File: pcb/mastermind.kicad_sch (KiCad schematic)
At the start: 14 parts, among them J1 Battery connector, SW1 SW_Push, SW2 SW_Push, SW3 SW_Push, SW4 SW_Push, SW5 SW_Push, SW6 SW_Push, SW7 SW_RST, U1 SuperMini nRF52840

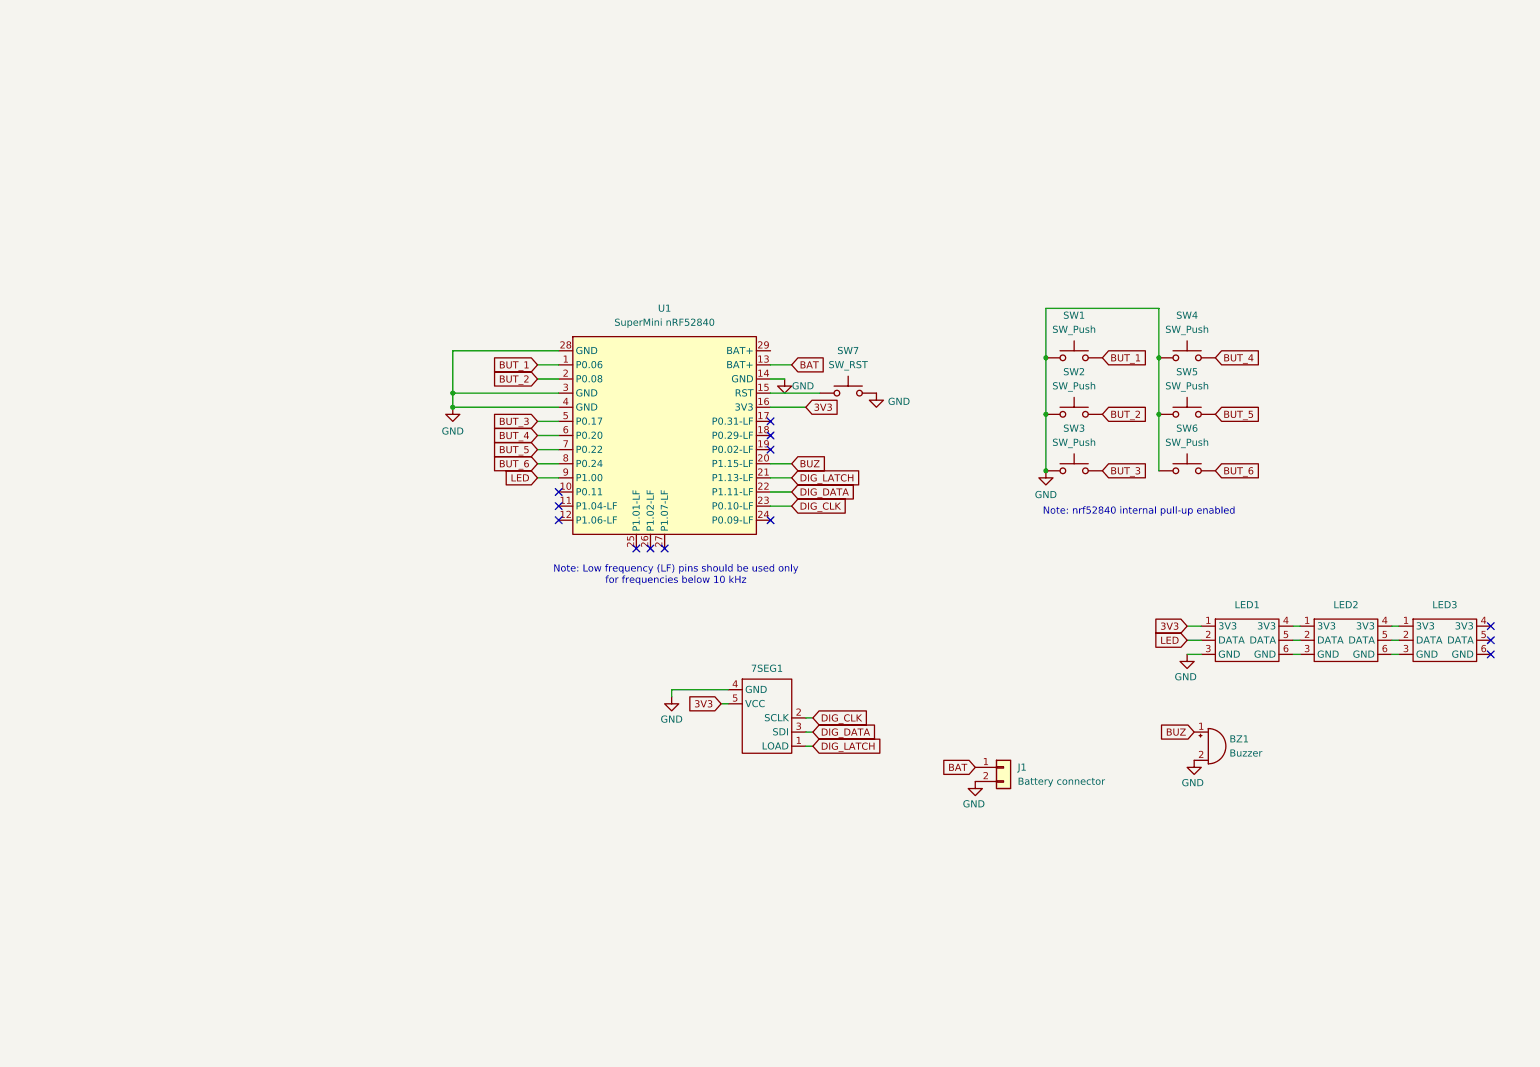
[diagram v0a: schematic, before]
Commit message: pcb: update files
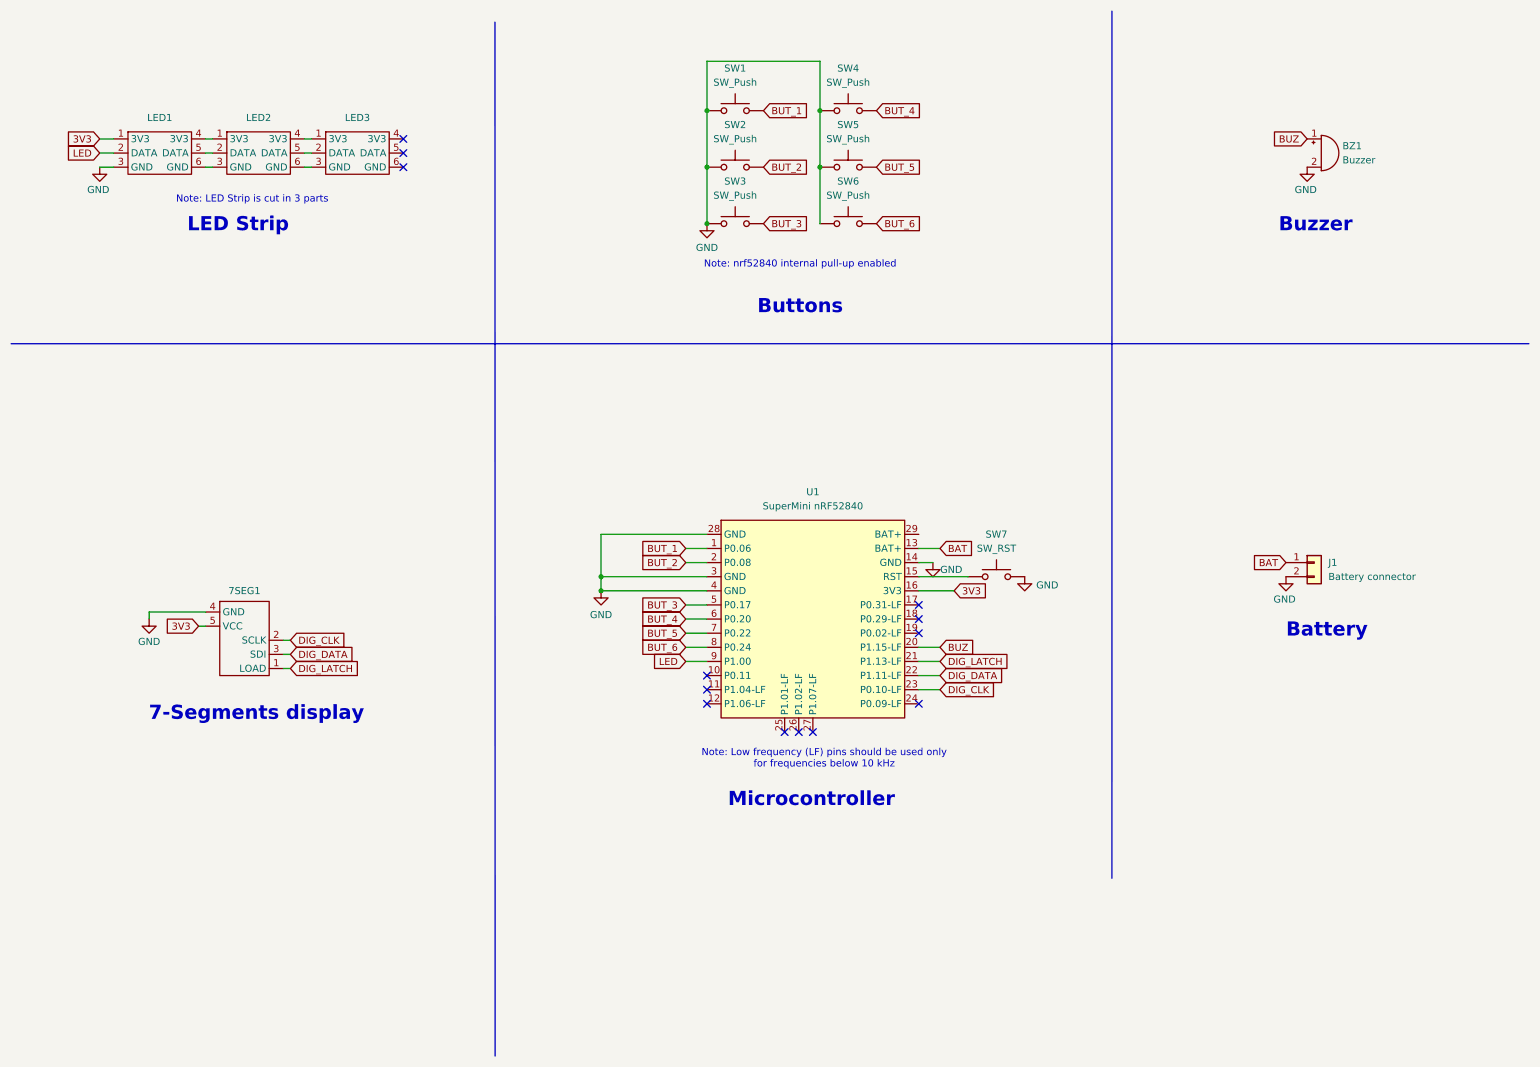
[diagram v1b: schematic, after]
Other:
- note added: "7-Segments display"
- note added: "Battery"
- note added: "Buttons"
- note added: "Buzzer"
- note added: "LED Strip"
- note added: "Microcontroller"
- note added: "Note: LED Strip is cut in 3 parts"
- moved on the sheet: 7SEG1, BZ1, J1, LED1, LED2, LED3, SW1, SW2, SW3, SW4, SW5, SW6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
